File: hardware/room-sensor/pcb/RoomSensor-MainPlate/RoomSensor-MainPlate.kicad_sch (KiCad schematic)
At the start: 10 parts

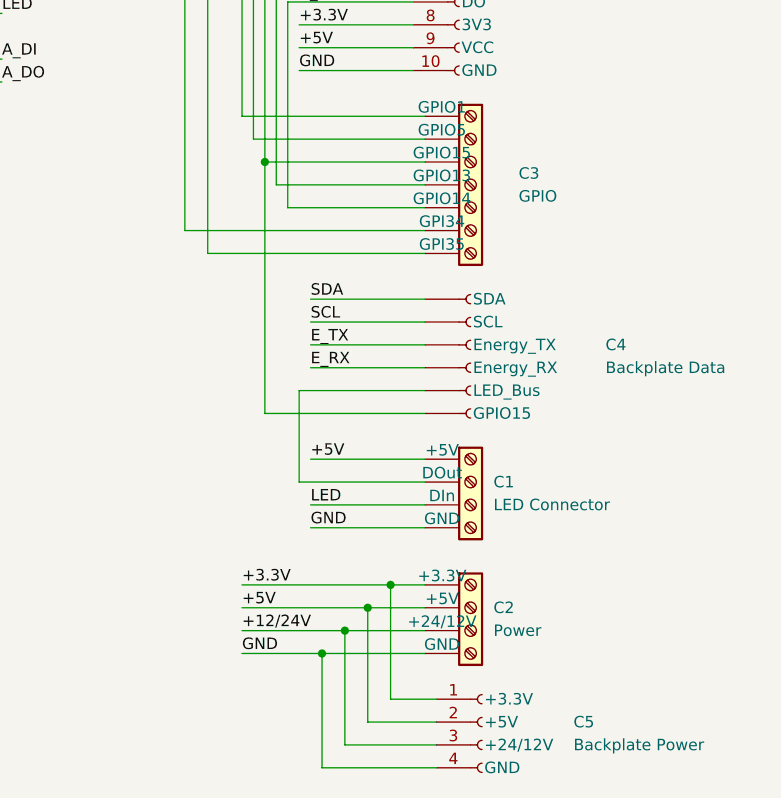
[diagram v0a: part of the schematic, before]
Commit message: PCB Design
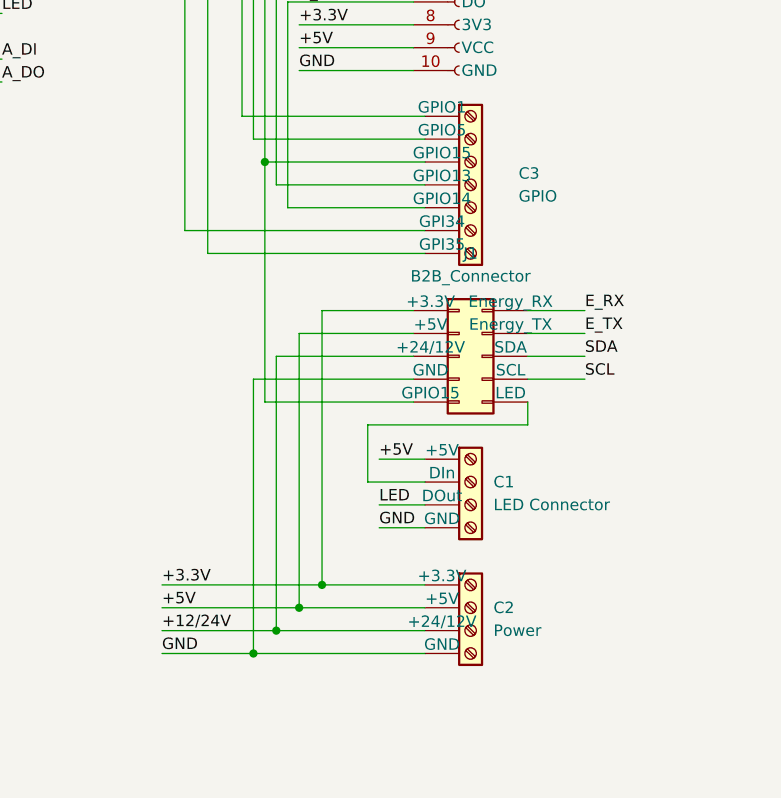
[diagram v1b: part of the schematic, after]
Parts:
- removed C4: Backplate Data, Connector_JST:JST_XH_B6B-XH-A_1x06_P2.50mm_Vertical, symbol Connector:Conn_01x06_Socket
- removed C5: Backplate Power, Connector_JST:JST_XH_B4B-XH-A_1x04_P2.50mm_Vertical, symbol Connector:Conn_01x04_Socket
- added J1: B2B_Connector, room-sensor:B2B Connector, symbol room-sensor:B2B_Connector
- A1: footprint Connector_PinSocket_2.54mm:PinSocket_1x10_P2.54mm_Vertical -> room-sensor:ES8311 + NS4150B Connector; MPN (none) -> 61301011821
- C1, C2: MPN (none) -> 1725672
- C3: MPN (none) -> 1725708
- E1: MPN (none) -> 61302621821
- S1: footprint Connector_PinSocket_2.54mm:PinSocket_1x05_P2.54mm_Vertical -> room-sensor:DFRobot C4002 Connector; MPN (none) -> 61300511821
- S2: footprint Connector_PinSocket_2.54mm:PinSocket_1x05_P2.54mm_Vertical -> room-sensor:BH1750; MPN (none) -> 61300511821
- S3: footprint Connector_PinSocket_2.54mm:PinSocket_1x08_P2.54mm_Vertical -> room-sensor:ENS160 + AHT20 Connector; MPN (none) -> 61300811821
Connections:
- net +12/24V: now also J1.5 (+24/12V)
- net +3.3V: now also J1.1 (+3.3V)
- net +5V: now also J1.3 (+5V)
- net A_DI: now also J1.9 (GPIO15)
- net E_RX: now also J1.2 (Energy_RX)
- net E_TX: now also J1.4 (Energy_TX)
- net GND: now also J1.7 (GND)
- net SCL: now also J1.8 (SCL)
- net SDA: now also J1.6 (SDA)
- net at C1.2 (DIn): now also J1.10 (LED)
